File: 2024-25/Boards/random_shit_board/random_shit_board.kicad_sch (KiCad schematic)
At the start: 7 parts, among them J1 043045-0212

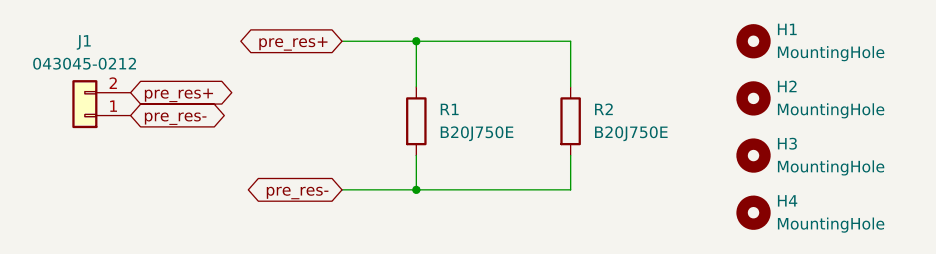
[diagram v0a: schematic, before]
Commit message: ESF changes
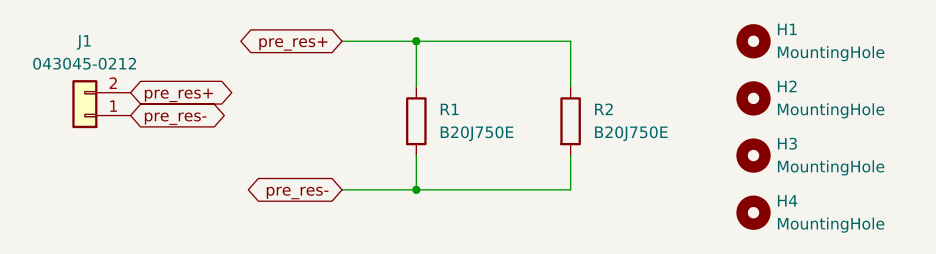
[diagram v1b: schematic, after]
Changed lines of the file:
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@@
 		(fields_autoplaced yes)
 		(property "Reference" "R1"
-			(at 119.38 72.39 0)
+			(at 119.38 72.3899 0)
 			(effects
 				(font
@@
 		)
 		(property "Value" "B20J750E"
-			(at 119.38 74.93 0)
+			(at 119.38 74.9299 0)
 			(effects
 				(font
